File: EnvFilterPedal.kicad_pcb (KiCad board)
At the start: 2 copper layers, 85 x 53 mm, 109 parts, among them J101 ScopeGroundLoop, J102 IO, Q101 BC857, Q102 BC857, U101 TL074, U102 TL074, U103 LM13700, U104 LM13700, U105 AZ34063U

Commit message: rev2 simulation stuff
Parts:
- C111, C113, C119, C120: value 1u -> 470n
- R103: value 470 -> 22k
- R110, R111: value 15k -> 6k8
- R121, R122, R124, R125: value 1k -> 680
- R130: value 4k7 -> 1k8
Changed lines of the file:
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@@
 			)
 		)
-		(property "Value" "1k"
+		(property "Value" "680"
 			(at 0 -1.65 0)
 			(layer "B.Fab")
@@
 			)
 		)
-		(property "Value" "1k"
+		(property "Value" "680"
 			(at 0 -1.65 0)
 			(layer "B.Fab")
@@
 			)
 		)
-		(property "Value" "1u"
+		(property "Value" "470n"
 			(at 0 -1.68 0)
 			(layer "B.Fab")
@@
 			)
 		)
-		(property "Value" "1u"
+		(property "Value" "470n"
 			(at 0 -1.679999 0)
 			(layer "B.Fab")
@@
 			)
 		)
-		(property "Value" "470"
+		(property "Value" "22k"
 			(at 0 -1.65 90)
 			(layer "B.Fab")
@@
 			)
 		)
-		(property "Value" "15k"
+		(property "Value" "6k8"
 			(at 0 -1.65 90)
 			(layer "B.Fab")
@@
 			)
 		)
-		(property "Value" "4k7"
+		(property "Value" "1k8"
 			(at 0 -1.65 0)
 			(layer "B.Fab")
@@
 			)
 		)
-		(property "Value" "15k"
+		(property "Value" "6k8"
 			(at 0 -1.65 90)
 			(layer "B.Fab")
@@
 			)
 		)
-		(property "Value" "1u"
+		(property "Value" "470n"
 			(at 0 -1.68 0)
 			(layer "B.Fab")
@@
 			)
 		)
-		(property "Value" "1u"
+		(property "Value" "470n"
 			(at 0 -1.679999 0)
 			(layer "B.Fab")
@@
 			)
 		)
-		(property "Value" "1k"
+		(property "Value" "680"
 			(at 0 -1.65 0)
 			(layer "B.Fab")
@@
 			)
 		)
-		(property "Value" "1k"
+		(property "Value" "680"
 			(at 0 -1.65 0)
 			(layer "B.Fab")

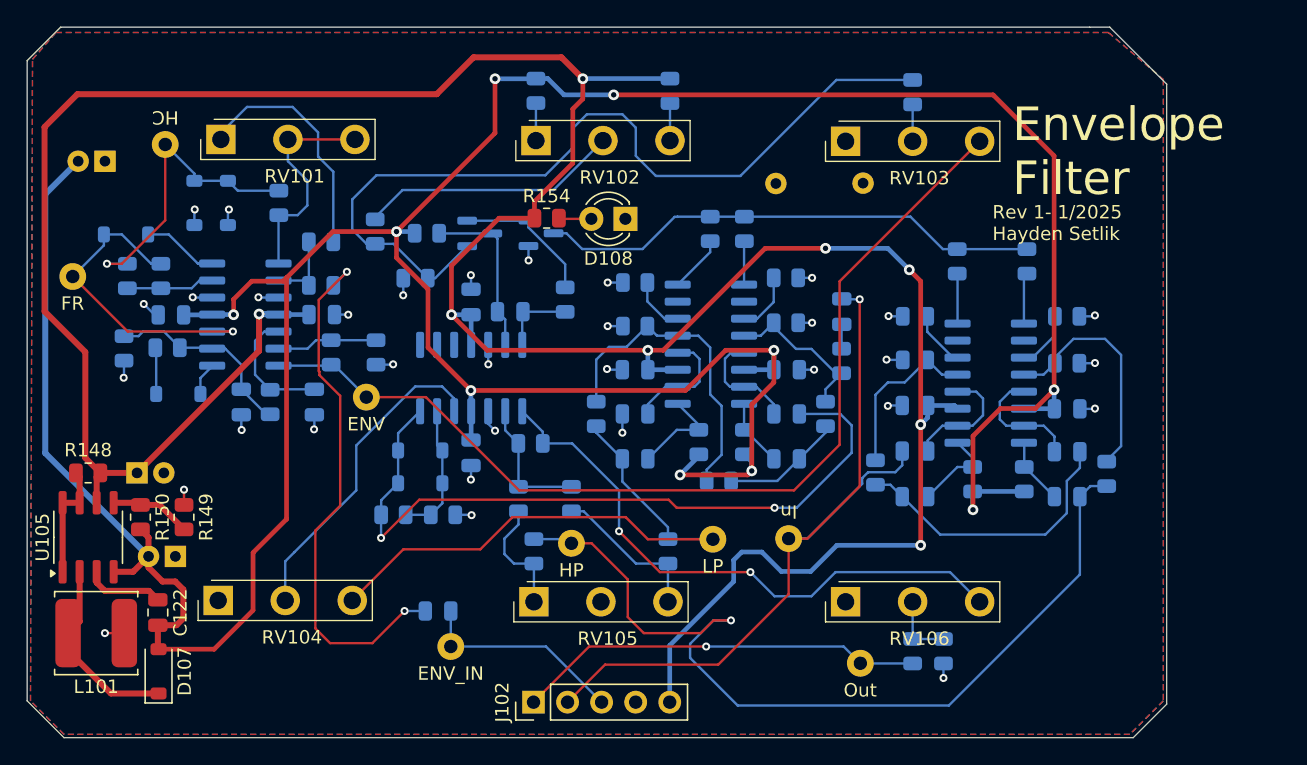
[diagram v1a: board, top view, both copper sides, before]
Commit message: 4 layer layout
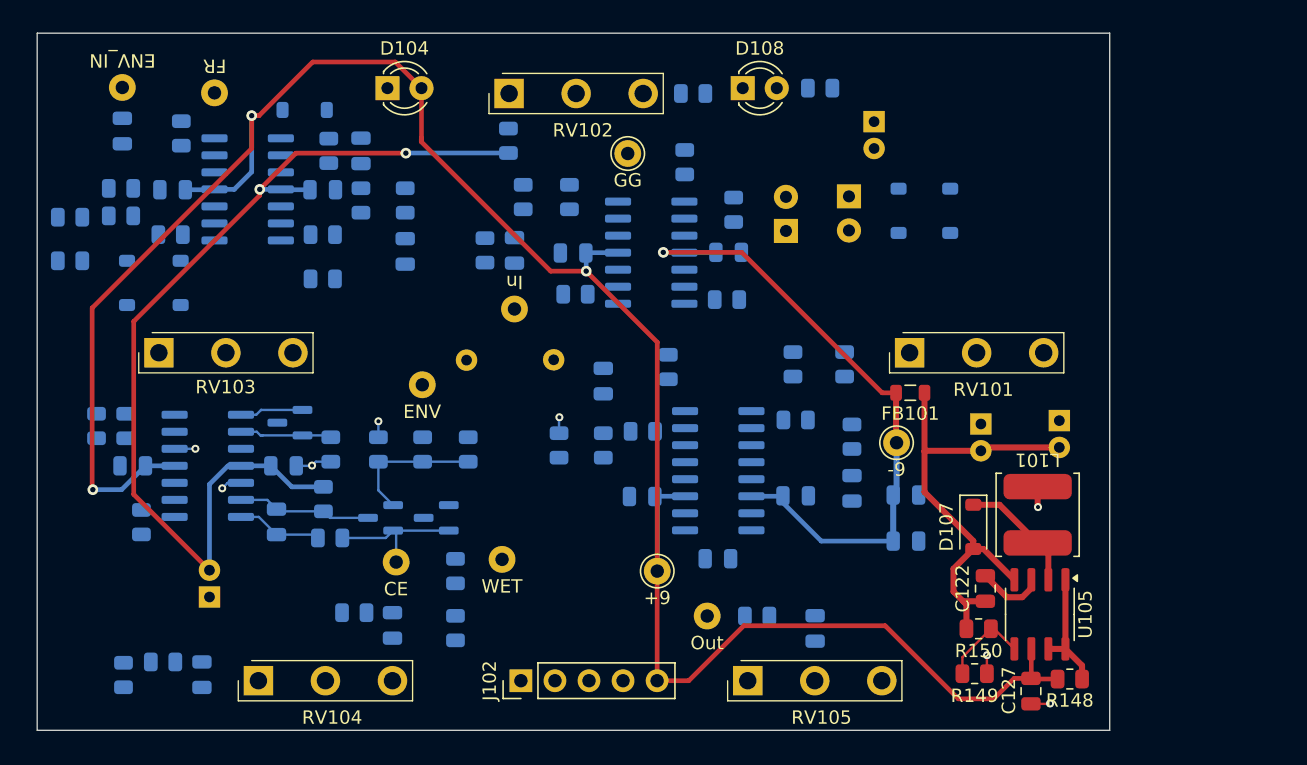
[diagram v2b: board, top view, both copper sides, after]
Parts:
- removed R144: 33k, Resistor_SMD:R_0805_2012Metric
- removed R145, R146, R151: 100k, Resistor_SMD:R_0805_2012Metric
- removed R147: 470, Resistor_SMD:R_0805_2012Metric
- removed RV106: 100kA, Potentiometer_THT:Potentiometer_Alpha_RV16AF_42_VeryLong
- added C126: 100n, Capacitor_SMD:C_0805_2012Metric, B.Cu at (68.8, 79.2)
- added C127: 22u, Capacitor_SMD:C_0805_2012Metric, F.Cu at (78.1, 93.8)
- added D109: 1N4148W, Diode_SMD:D_SOD-123, B.Cu at (68.2, 58.0)
- added D110: 1N4148W, Diode_SMD:D_SOD-123, B.Cu at (72.1, 58.0)
- added FB101: 90R, Inductor_SMD:L_0805_2012Metric, F.Cu at (69.1, 71.5)
- added Q103: BC847, Package_TO_SOT_SMD:SOT-23, B.Cu at (22.9, 73.8)
- added TP109: +9, TestPoint:TestPoint_THTPad_D2.0mm_Drill1.0mm_VAL, F.Cu at (50.2, 84.8)
- added TP110: -9, TestPoint:TestPoint_THTPad_D2.0mm_Drill1.0mm_VAL, F.Cu at (68.1, 75.2)
- C105: value 100n -> 470u; footprint Capacitor_SMD:C_0805_2012Metric -> Capacitor_THT:CP_Radial_D5.0mm_P2.00mm
- C109: value 100n -> 1u
- C110: value 1n -> 10n
- C111: value 470n -> 100n
- C112: value 1n -> 100n
- C113, C119, C120: value 470n -> 1u
- C116: value 1u -> 1n
- C118: value 1n -> 1u
- C125: value 10n -> 1u
- D104: value 1N4148W -> LED; footprint Diode_SMD:D_SOD-123 -> LED_THT:LED_D3.0mm; moved to F.Cu
- D105, D106: value 1N4148W -> LED; footprint Diode_SMD:D_SOD-123 -> LED_THT:LED_D3.0mm
- R101, R103, R118: value 22k -> 100k
- R102: value 47k -> 100k
- R106, R125: value 680 -> 1k
- R109: value 22k -> 6k8
- R117: value 4k7 -> 100k
- R119: value 33k -> 1k8
- R120: value 33k -> 100k
- R121: value 680 -> 1M
- R122: value 680 -> 47k
- R123: value 33k -> 12k
- R124: value 680 -> 100k
- R126: value 4k7 -> 1k
- R128, R132: value 22k -> 33k
- R129: value 10k -> 1k
- R130: value 1k8 -> 1k
- R131: value 4k7 -> 33k
- R133: value 33k -> 4k7
- R134: value 1k -> 4k7
- R135: value 1k -> 10k
- R136: value 1k -> 1k8
- R137: value 1k -> 470k
- R138: value 33k -> 1Meg
- R139: value 4k7 -> 470k
- R140: value 22k -> 1Meg
- R143: value 33k -> 220
- R154: moved to B.Cu
- RV104: value 10kB -> 100kB
- RV105: value 100kB -> 100kA
- TP103: value HP -> CE
- TP104: value LP -> WET
- TP107: value HC -> GG; moved to F.Cu
- U103: value LM13700 -> TL074; footprint Package_SO:SOIC-16_3.9x9.9mm_P1.27mm -> Package_SO:SOIC-14_3.9x8.7mm_P1.27mm
- moved R138 74.9 mm to (10.4, 92.6)
- moved R148 74.8 mm to (81.0, 92.9), turned to 0 degrees
- moved C124 73.8 mm to (80.2, 73.6), turned to -90 degrees
- moved R137 72.2 mm to (13.4, 91.6)
- moved U105 71.2 mm to (78.8, 88.0), turned to -90 degrees
- moved L101 70.8 mm to (78.6, 80.6), turned to 90 degrees
- moved R140 65.9 mm to (11.8, 81.2)
- moved R150 63.1 mm to (74.2, 89.1), turned to 180 degrees
- moved C122 61.8 mm to (74.7, 86.1)
- moved D107 61.7 mm to (73.8, 81.5), turned to -90 degrees
- moved C121 60.9 mm to (66.4, 51.3), turned to -90 degrees
- moved C123 60.9 mm to (74.4, 73.8), turned to -90 degrees
- moved R149 60.1 mm to (73.9, 92.5), turned to 180 degrees
- moved R139 56.6 mm to (27.6, 87.9), turned to 180 degrees
- moved R120 55.3 mm to (10.2, 56.3), turned to 180 degrees
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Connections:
- C104 pad 1: /EnvCap -> Net-(U101C--)
- C105 pad 1: +9V -> GND
- C105 pad 2: GND -> -9V
- C106 pad 1: -9V -> +9V
- C108 pad 1: +9V -> -9V
- C109 pad 1: -9V -> FX_IN
- C109 pad 2: GND -> Net-(U103B-+)
- C110 pad 1: Net-(C110-Pad1) -> Net-(U101D-+)
- C110 pad 2: Net-(D105-A) -> GND
- C111 pad 1: Net-(C111-Pad1) -> +9V
- C111 pad 2: Net-(C111-Pad2) -> GND
- C112 pad 1: Net-(C112-Pad1) -> -9V
- C113 pad 1: Net-(C113-Pad1) -> /GTR_GAIN
- C113 pad 2: LP_OUT -> Net-(C113-Pad2)
- C116 pad 1: FX_IN -> Net-(U103D-+)
- C116 pad 2: Net-(C116-Pad2) -> GND
- C117 pad 1: Net-(C117-Pad1) -> Net-(U103A-+)
- C117 pad 2: FX_IN -> Net-(D105-A)
- C118 pad 2: /HP1 -> Net-(C118-Pad2)
- C119 pad 2: /HP1 -> Net-(C119-Pad2)
- C120 pad 2: HP_OUT -> Net-(C120-Pad2)
- C122 pad 2: -9V -> Net-(D107-A)
- C123 pad 2: -9V -> Net-(D107-A)
- C124 pad 2: -9V -> Net-(D107-A)
- C125 pad 1: Net-(U101B-+) -> -9V
- D101 pad 1: GND -> Net-(D101-K)
- D101 pad 2: /HardClip -> Net-(D101-A)
- D102 pad 1: /HardClip -> Net-(D101-A)
- D102 pad 2: GND -> Net-(D102-A)
- D103 pad 1: /FullRect -> Net-(D103-K)
- D104 pad 2: Net-(D104-A) -> +9V
- D107 pad 2: -9V -> Net-(D107-A)
- R101 pad 1: Net-(C103-Pad2) -> Net-(D102-A)
- R101 pad 2: Net-(U101A--) -> Net-(U101B--)
- R102 pad 1: Net-(U101A--) -> Net-(D102-A)
- R102 pad 2: Net-(R102-Pad2) -> Net-(U101B--)
- R103 pad 1: Net-(R103-Pad1) -> Net-(U101B--)
- R103 pad 2: /HardClip -> /FullRect
- R104 pad 1: /HardClip -> Net-(C103-Pad2)
- R104 pad 2: Net-(U101D--) -> Net-(D101-K)
- R105 pad 1: Net-(U101D--) -> Net-(D101-K)
- R105 pad 2: /FullRect -> Net-(D102-A)
- R106 pad 1: Net-(D104-K) -> Net-(D103-K)
- R106 pad 2: /EnvCap -> Net-(U101C--)
- R107 pad 1: /EnvCap -> Net-(U101C--)
- R108 pad 1: Net-(U101B--) -> Net-(U101D--)
- R108 pad 2: ENV -> /EnvPos
- R109 pad 1: Net-(U101B--) -> Net-(U101D--)
- R112 pad 1: Net-(R112-Pad1) -> ENV
- R117 pad 1: Net-(R117-Pad1) -> /EnvPos
- R117 pad 2: Iabc -> Net-(U102B--)
- R118 pad 1: Net-(C111-Pad1) -> Net-(U102B--)
- R118 pad 2: -9V -> /EnvNeg
- R119 pad 1: Net-(U103C--) -> Net-(Q103-E)
- R119 pad 2: Net-(C111-Pad2) -> GND
- R120 pad 1: Net-(C116-Pad2) -> Net-(C103-Pad2)
- R120 pad 2: Net-(U103C--) -> Net-(U101B--)
- R121 pad 1: GND -> Net-(U103B-+)
- R121 pad 2: Net-(U103C--) -> GND
- R122 pad 1: GND -> Net-(U103B--)
- R122 pad 2: Net-(U103C-+) -> /GTR_GAIN
- R123 pad 1: Net-(C111-Pad2) -> Net-(U103B--)
- R123 pad 2: Net-(U103A--) -> GND
- R124 pad 1: GND -> Net-(U101C--)
- R124 pad 2: Net-(U103A--) -> Net-(U101D-+)
- R125 pad 2: Net-(U103A-+) -> Net-(U104A--)
- R126 pad 1: Net-(R126-Pad1) -> GND
- R126 pad 2: Iabc -> Net-(U104A-+)
- R127 pad 1: Net-(U103A--) -> Net-(C113-Pad2)
- R127 pad 2: LP_OUT -> Net-(U104A--)
- R128 pad 1: Net-(C113-Pad1) -> Net-(U104A--)
- R128 pad 2: -9V -> Net-(U103A--)
- R129 pad 1: Net-(D105-A) -> GND
- R129 pad 2: Net-(D105-K) -> Net-(U104C--)
- R130 pad 1: Net-(D105-K) -> GND
- R130 pad 2: GND -> Net-(U104C-+)
- R131 pad 1: Iabc -> Net-(U103A--)
- R131 pad 2: Net-(R131-Pad2) -> Net-(U104C-+)
- R132 pad 1: Net-(C119-Pad1) -> Net-(U104C--)
- R132 pad 2: -9V -> /WET
- R133 pad 1: Net-(U104A--) -> Iabc
- R133 pad 2: /HP1 -> Net-(R133-Pad2)
- R134 pad 1: GND -> Iabc
- R134 pad 2: Net-(U104A-+) -> Net-(R134-Pad2)
- R135 pad 1: GND -> Net-(D105-A)
- R135 pad 2: Net-(U104A--) -> Net-(D105-K)
- R136 pad 2: Net-(U104C--) -> Net-(D105-K)
- R137 pad 1: GND -> Net-(C119-Pad2)
- R137 pad 2: Net-(U104C-+) -> Net-(U102A-+)
- R138 pad 1: Net-(U104C--) -> Net-(U102A-+)
- R138 pad 2: HP_OUT -> GND
- R139 pad 1: Iabc -> Net-(C118-Pad2)
- R139 pad 2: Net-(R139-Pad2) -> Net-(U102A--)
- R140 pad 1: Net-(C120-Pad1) -> Net-(U102A--)
- R140 pad 2: -9V -> Net-(R140-Pad2)
- R141 pad 1: HP_OUT -> /WET
- R141 pad 2: Net-(R141-Pad2) -> Net-(C119-Pad1)
- R142 pad 1: LP_OUT -> /GTR_GAIN
- R142 pad 2: Net-(R142-Pad2) -> Net-(C118-Pad1)
- R143 pad 1: Net-(R141-Pad2) -> Net-(C120-Pad1)
- R143 pad 2: Net-(U102C--) -> FX_OUT
- R150 pad 2: -9V -> Net-(D107-A)
- RV101 pad 1: Net-(R102-Pad2) -> GND
- RV101 pad 2: Net-(R103-Pad1) -> Net-(U103C-+)
- RV101 pad 3: Net-(R103-Pad1) -> /WET
- RV103 pad 1: GND -> /EnvNeg
- RV103 pad 2: Net-(R112-Pad1) -> ENV
- RV103 pad 3: ENV -> /EnvPos
- RV104 pad 1: GND -> Net-(C119-Pad1)
- RV104 pad 2: Net-(U102D-+) -> GND
- RV104 pad 3: LP_OUT -> Net-(C118-Pad1)
- RV105 pad 1: Net-(R141-Pad2) -> GND
- RV105 pad 2: GND -> Net-(C120-Pad2)
- RV105 pad 3: Net-(R142-Pad2) -> Net-(R140-Pad2)
- TP103 pad 1: HP_OUT -> /ComEmmiter
- TP104 pad 1: LP_OUT -> /WET
- TP107 pad 1: /HardClip -> /GTR_GAIN
- U101 pad 1: Net-(R103-Pad1) -> Net-(D101-A)
- U101 pad 12: GND -> Net-(U101D-+)
- U101 pad 14: Net-(D103-A) -> /EnvPos
- U101 pad 2: Net-(U101A--) -> Net-(D101-K)
- U101 pad 5: Net-(U101B-+) -> GND
- U101 pad 7: ENV -> /FullRect
- U101 pad 8: Net-(D104-A) -> Net-(D103-A)
- U101 pad 9: /EnvCap -> Net-(U101C--)
- U102 pad 1: unconnected-(U102-Pad1) -> Net-(R140-Pad2)
- U102 pad 10: GND -> /EnvPos
- U102 pad 12: Net-(U102D-+) -> GND
- U102 pad 13: Net-(D105-K) -> Net-(Q102-C)
- U102 pad 14: Net-(D105-A) -> Net-(C107-Pad1)
- U102 pad 2: unconnected-(U102A---Pad2) -> Net-(U102A--)
- U102 pad 3: unconnected-(U102A-+-Pad3) -> Net-(U102A-+)
- U102 pad 6: Net-(Q102-C) -> Net-(U102B--)
- U102 pad 7: Net-(C107-Pad1) -> /EnvNeg
- U102 pad 9: Net-(U102C--) -> Net-(Q103-E)
- U103 pad 1: Net-(R117-Pad1) -> Net-(U103A--)
- U103 pad 10: Net-(C112-Pad1) -> Net-(U103C-+)
- U103 pad 11: +9V -> -9V
- U103 pad 12: Net-(C112-Pad1) -> Net-(U103D-+)
- U103 pad 13: Net-(U103A--) -> /WET
- U103 pad 14: Net-(U103A-+) -> /WET
- U103 pad 2: unconnected-(U103C-DIODE_BIAS-Pad2) -> Net-(U103A--)
- U103 pad 3: Net-(U103C-+) -> Net-(U103A-+)
- U103 pad 4: Net-(U103C--) -> +9V
- U103 pad 5: Net-(C110-Pad1) -> Net-(U103B-+)
- U103 pad 6: -9V -> Net-(U103B--)
- U103 pad 7: Net-(C110-Pad1) -> /GTR_GAIN
- U103 pad 8: Net-(C111-Pad1) -> Net-(D105-A)
- U103 pad 9: Net-(C113-Pad1) -> Net-(D105-K)
- U104 pad 1: Net-(R139-Pad2) -> Net-(R134-Pad2)
- U104 pad 10: Net-(C117-Pad1) -> unconnected-(U104-Pad10)
- U104 pad 12: Net-(C117-Pad1) -> Net-(U103A-+)
- U104 pad 16: Net-(R131-Pad2) -> Net-(R133-Pad2)
- U104 pad 5: Net-(C118-Pad1) -> Net-(U103D-+)
- U104 pad 7: Net-(C118-Pad1) -> unconnected-(U104-Pad7)
- U104 pad 8: Net-(C120-Pad1) -> unconnected-(U104-Pad8)
- U104 pad 9: Net-(C119-Pad1) -> unconnected-(U104-Pad9)
- U105 pad 4: -9V -> Net-(D107-A)
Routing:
- net -9V: track 265.9 -> 123.6 mm, vias 10 -> 3
- net ENV: track 74.1 -> 0.00 mm
- net HP_OUT: track 67.2 -> 0.00 mm, vias 1 -> 0
- net FX_IN: track 58.2 -> 0.00 mm, vias 1 -> 0
- net +9V: track 224.1 -> 165.9 mm, vias 8 -> 3
- net Net-(D105-A): track 55.2 -> 0.00 mm, vias 2 -> 0
- net /vBase: track 64.7 -> 10.4 mm
- net LP_OUT: track 44.2 -> 0.00 mm
- net Net-(C103-Pad2): track 40.0 -> 0.00 mm, vias 2 -> 0
- net Net-(Q103-B): track 43.8 -> 4.74 mm, vias 2 -> 0
- net Iabc: track 37.8 -> 0.00 mm
- net Net-(D107-A): track 0.00 -> 36.0 mm
- net FX_OUT: track 30.5 -> 0.00 mm, vias 1 -> 0
- net GND: track 40.0 -> 12.6 mm, vias 33 -> 8
- net /FullRect: track 24.5 -> 0.00 mm, vias 1 -> 0
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- added copper zone on In1.Cu, net GND
- added copper zone on In2.Cu, net GND
- removed copper zone on B.Cu, net GND
- removed copper zone on F.Cu, net GND
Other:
- board size 85 x 53 mm -> 80 x 52 mm
- copper layers 2 -> 4
- board text removed: "Envelope Filter"
- board text removed: "Rev 1- 1/2025 Hayden Setlik"
